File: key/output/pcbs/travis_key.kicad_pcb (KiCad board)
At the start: 2 copper layers, 38.1 x 38.1 mm, 4 parts

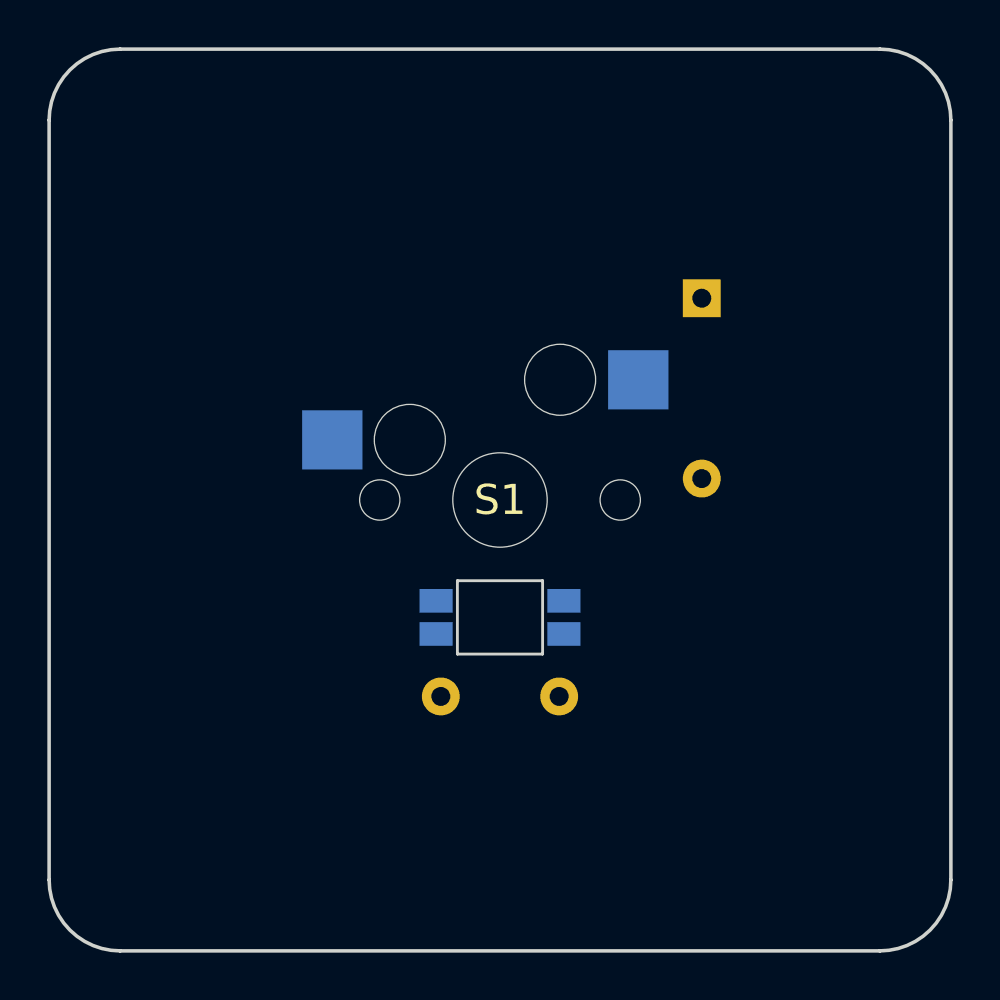
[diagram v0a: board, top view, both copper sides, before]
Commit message: footprint wip
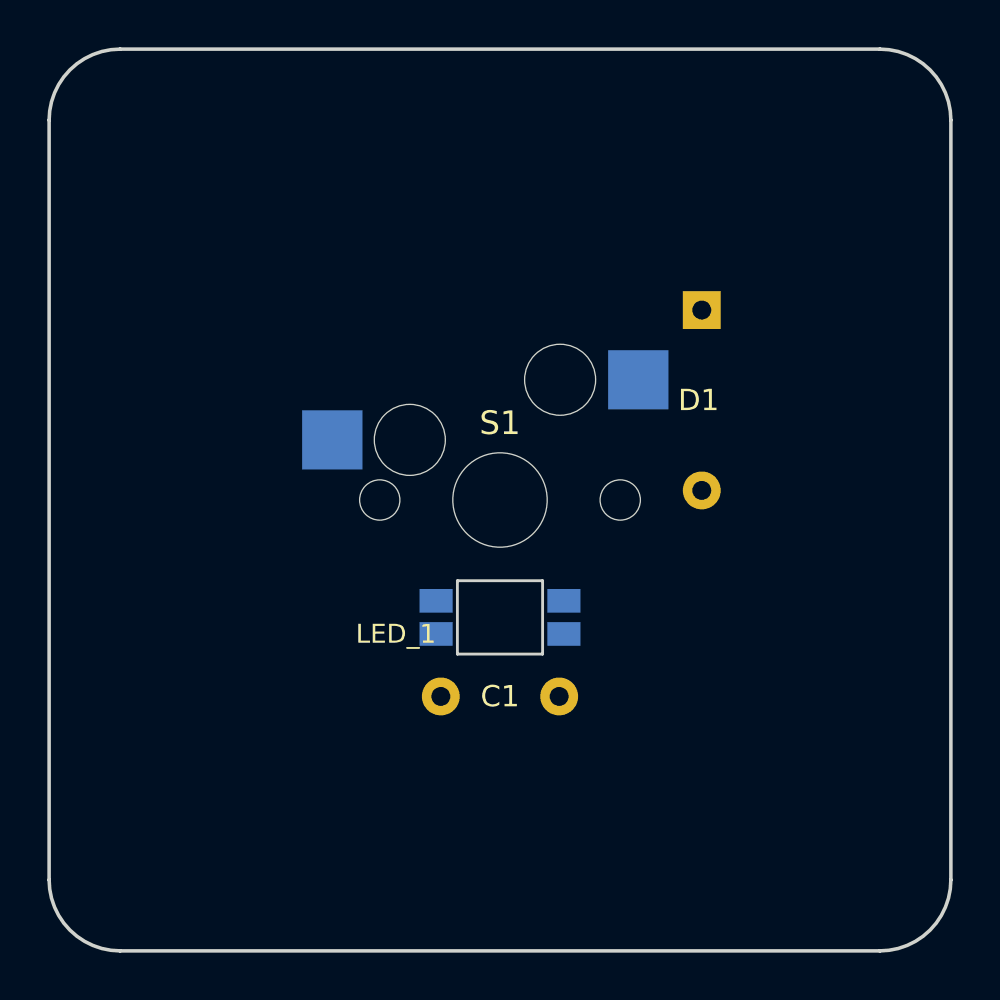
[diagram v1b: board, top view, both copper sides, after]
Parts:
- LED1: value (none) -> SK6812mini-e; footprint ceoloide:led_SK6812mini-e (per-keysingle-side) -> ceoloide:led_SK6812mini-e (per-key single-side)
- S1: value (none) -> Kailh MX Switch Sockets
- moved D1 0.50 mm to (8.53, -8.03)
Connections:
- net LED_0 renamed LED_2
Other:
- board text added: "C1"
- board text added: "D1"
- board text added: "LED_1"
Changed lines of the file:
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@@
   (title_block
     (title travis_key)
-    (rev 2024.03.20)
+    (rev 2024.03.23)
     (company "Travis Hardiman")
   )
@@
 (net 3 "row0")
 (net 4 "RAW")
-(net 5 "LED_0")
+(net 5 "LED_2")
 (net 6 "GND")
 (net 7 "LED_1")
@@
 (add_net "row0")
 (add_net "RAW")
-(add_net "LED_0")
+(add_net "LED_2")
 (add_net "GND")
 (add_net "LED_1")
   )
-      (module MX (layer F.Cu)
-      (at 0 0 0)
-      (fp_text reference "S1" (at 0 0) (layer F.SilkS)  (effects (font (size 1.27 1.27) (thickness 0.15))))
-      (fp_text value "" (at 0 0) (layer F.SilkS) hide (effects (font (size 1.27 1.27) (thickness 0.15))))
-      (fp_line (start -7 -6) (end -7 -7) (layer Dwgs.User) (width 0.15))
-      (fp_line (start -7 7) (end -6 7) (layer Dwgs.User) (width 0.15))
-      (fp_line (start -6 -7) (end -7 -7) (layer Dwgs.User) (width 0.15))
-      (fp_line (start -7 7) (end -7 6) (layer Dwgs.User) (width 0.15))
-      (fp_line (start 7 6) (end 7 7) (layer Dwgs.User) (width 0.15))
-      (fp_line (start 7 -7) (end 6 -7) (layer Dwgs.User) (width 0.15))
-      (fp_line (start 6 7) (end 7 7) (layer Dwgs.User) (width 0.15))
-      (fp_line (start 7 -7) (end 7 -6) (layer Dwgs.User) (width 0.15))
-      (pad "" np_thru_hole circle (at 0 0) (size 3.9878 3.9878) (drill 3.9878) (layers *.Cu *.Mask))
-      (pad "" np_thru_hole circle (at 5.08 0) (size 1.7018 1.7018) (drill 1.7018) (layers *.Cu *.Mask))
-      (pad "" np_thru_hole circle (at -5.08 0) (size 1.7018 1.7018) (drill 1.7018) (layers *.Cu *.Mask))
-      (fp_line (start -9.5 -9.5) (end 9.5 -9.5) (layer Dwgs.User) (width 0.15))
-      (fp_line (start 9.5 -9.5) (end 9.5 9.5) (layer Dwgs.User) (width 0.15))
-      (fp_line (start 9.5 9.5) (end -9.5 9.5) (layer Dwgs.User) (width 0.15))
-      (fp_line (start -9.5 9.5) (end -9.5 -9.5) (layer Dwgs.User) (width 0.15))
-        (pad "" np_thru_hole circle (at 2.54 -5.08) (size 3 3) (drill 3) (layers *.Cu *.Mask))
-        (pad "" np_thru_hole circle (at -3.81 -2.54) (size 3 3) (drill 3) (layers *.Cu *.Mask))
-        (pad 1 smd rect (at -7.085 -2.54 0) (size 2.55 2.5) (layers B.Cu B.Paste B.Mask) (net 1 "col0"))
-        (pad 2 smd rect (at 5.842 -5.08 0) (size 2.55 2.5) (layers B.Cu B.Paste B.Mask) (net 2 "single_A_one"))
-        )
+        (module MX (layer F.Cu)
+        (at 0 0 0)
+        (fp_text reference "S1" (at 0 -3.25) (layer F.SilkS)  (effects (font (size 1 1) (thickness 0.15))))
+        (fp_text value "Kailh MX Switch Sockets" (at 0 0) (layer B.Fab) hide (effects (font (size 1 1) (thickness 0.15))))
+        (fp_line (start -7 -6) (end -7 -7) (layer Dwgs.User) (width 0.15))
+        (fp_line (start -7 7) (end -6 7) (layer Dwgs.User) (width 0.15))
+        (fp_line (start -6 -7) (end -7 -7) (layer Dwgs.User) (width 0.15))
+        (fp_line (start -7 7) (end -7 6) (layer Dwgs.User) (width 0.15))
+        (fp_line (start 7 6) (end 7 7) (layer Dwgs.User) (width 0.15))
+        (fp_line (start 7 -7) (end 6 -7) (layer Dwgs.User) (width 0.15))
+        (fp_line (start 6 7) (end 7 7) (layer Dwgs.User) (width 0.15))
+        (fp_line (start 7 -7) (end 7 -6) (layer Dwgs.User) (width 0.15))
+        (pad "" np_thru_hole circle (at 0 0) (size 3.9878 3.9878) (drill 3.9878) (layers *.Cu *.Mask))
+        (pad "" np_thru_hole circle (at 5.08 0) (size 1.7018 1.7018) (drill 1.7018) (layers *.Cu *.Mask))
+        (pad "" np_thru_hole circle (at -5.08 0) (size 1.7018 1.7018) (drill 1.7018) (layers *.Cu *.Mask))
+        (fp_line (start -9.5 -9.5) (end 9.5 -9.5) (layer Dwgs.User) (width 0.15))
+        (fp_line (start 9.5 -9.5) (end 9.5 9.5) (layer Dwgs.User) (width 0.15))
+        (fp_line (start 9.5 9.5) (end -9.5 9.5) (layer Dwgs.User) (width 0.15))
+        (fp_line (start -9.5 9.5) (end -9.5 -9.5) (layer Dwgs.User) (width 0.15))
+          (pad "" np_thru_hole circle (at 2.54 -5.08) (size 3 3) (drill 3) (layers *.Cu *.Mask))
+          (pad "" np_thru_hole circle (at -3.81 -2.54) (size 3 3) (drill 3) (layers *.Cu *.Mask))
+          (pad 1 smd rect (at -7.085 -2.54 0) (size 2.55 2.5) (layers B.Cu B.Paste B.Mask) (net 1 "col0"))
+          (pad 2 smd rect (at 5.842 -5.08 0) (size 2.55 2.5) (layers B.Cu B.Paste B.Mask) (net 2 "single_A_one"))
+      (model "${SCOTTOKEEBS_KICAD}/3dmodels/ScottoKeebs_Hotswap.3dshapes/Hotswap_MX.step"
+		(offset (xyz 0 0 0) )
+		(scale (xyz 1 1 1) )
+		(rotate (xyz 0 0 0) )
+	  ))
     (module "Diode_DO-35" (layer "B.Cu")
     (descr "Diode, DO-35_SOD27 series, Axial, Horizontal, pin pitch=7.62mm, , length*diameter=4*2mm^2, , http://www.diodes.com/_files/packages/DO-35.pdf")
     (tags "Diode DO-35_SOD27 series Axial Horizontal pin pitch 7.62mm  length 4mm diameter 2mm")
-    (at 8.525 -8.525 270)
-    (fp_text reference "D1" (at 3.81 -2.12 270) (layer "B.SilkS")
+    (at 8.525 -8.025 270)
+    (fp_text reference "D1" (at 5.985 1.921 270) (layer "B.SilkS")
       (effects (font (size 1 1) (thickness 0.15)) (justify mirror))
     )
-    (fp_text value "1N4148" (at 3.81 0 270) (layer "B.Fab")
-      (effects (font (size 0.8 1) (thickness 0.15)))
-    )
-    (fp_text user "K" (at 0 -1.8 270) (layer "B.SilkS")
-      (effects (font (size 1 1) (thickness 0.15)) (justify mirror))
-    )
-    (fp_text user "K" (at 0 -1.8 270) (layer "B.Fab")
-      (effects (font (size 1 1) (thickness 0.15)) (justify mirror))
+    (fp_text value "1N4148" (at 11.065 0 270) (layer "B.Fab")
+      (effects (font (size 0.8 0.8) (thickness 0.15)))
     )
     (fp_line (start 1.04 0) (end 1.69 0)
@@
     )
   )
-      (module "ceoloide:led_SK6812mini-e (per-keysingle-side)"
+      (gr_text "D1" (at 7.525 -4.215 0) (layer F.SilkS)
+        (effects (font (size 0.9 0.9) (thickness 0.15)) (justify left))
+      )
+      (module "ceoloide:led_SK6812mini-e (per-key single-side)"
         (layer B.Cu)
         (at 0 4.96 0)
-        (fp_text reference "LED1" (at -4.75 0 90) (layer B.SilkS)
-          (effects (font (size 1 1) (thickness 0.15)))
+        (fp_text reference "LED1" (at -5.25 0 90) (layer B.SilkS)
+          (effects (font (size 1 1) (thickness 0.15)) (justify  mirror))
+        )
+        (fp_text value "SK6812mini-e" (at 0 -2.25 0) (layer "B.Fab")
+          (effects (font (size 0.8 0.8) (thickness 0.15)))
         )
         (fp_line (start -1.6 -1.4) (end 1.6 -1.4) (layer Dwgs.User) (width 0.12))
@@
         (fp_line (start -3.8 -1.6) (end -2.2 -1.6) (layer B.SilkS) (width 0.12))
         (fp_line (start -3.8 0) (end -3.8 -1.6) (layer B.SilkS) (width 0.12))
-        (pad 2 smd rect (at 2.70 -0.7 0) (size 1.4 1) (layers B.Cu B.Paste B.Mask) (net 5 "LED_0"))
+        (fp_line (start -3.8 -1.36) (end -3.56 -1.6) (layer B.SilkS) (width 0.12))
+        (pad 2 smd rect (at 2.70 -0.7 0) (size 1.4 1) (layers B.Cu B.Paste B.Mask) (net 5 "LED_2"))
         (pad 1 smd rect (at 2.70 0.7 0) (size 1.4 1) (layers B.Cu B.Paste B.Mask) (net 4 "RAW"))
         (pad 3 smd rect (at -2.70 -0.7 0) (size 1.4 1) (layers B.Cu B.Paste B.Mask) (net 6 "GND"))
@@
         )
       )
+      (gr_text "LED_1" (at -2.7 5.66 0) (layer F.SilkS)
+        (effects (font (size 0.8 0.8) (thickness 0.15)) (justify right))
+      )
     (module C_Disc_D4.7mm_W2.5mm_P5.00mm (layer B.Cu)
     (descr "C, Disc series, Radial, pin pitch=5.00mm, , diameter*width=4.7*2.5mm^2, Capacitor, http://www.vishay.com/docs/45233/krseries.pdf")
     (tags "C Disc series Radial pin pitch 5.00mm  diameter 4.7mm width 2.5mm Capacitor")
     (at 2.5 8.3 180)
-    (fp_text reference "C1" (at 2.5 -2.5 180) (layer B.SilkS)
+    (fp_text reference "C1" (at 7.5 0 180) (layer B.SilkS)
       (effects (font (size 1 1) (thickness 0.15)) (justify mirror))
     )
-    (fp_text value "104" (at 2.5 2.5 180) (layer B.Fab)
+    (fp_text value "104" (at -2.5 0 180) (layer B.Fab)
       (effects (font (size 1 1) (thickness 0.15)))
     )
@@
     (pad 1 thru_hole circle (at 0 0) (size 1.6 1.6) (drill 0.8) (layers *.Cu *.Mask) (net 4 "RAW"))
     (pad 2 thru_hole circle (at 5 0) (size 1.6 1.6) (drill 0.8) (layers *.Cu *.Mask) (net 6 "GND"))
-    (fp_text user %R (at 2.5 0) (layer B.Fab)
-      (effects (font (size 0.94 0.94) (thickness 0.141)))
-    )
     (model ${KISYS3DMOD}/Capacitor_THT.3dshapes/C_Disc_D4.7mm_W2.5mm_P5.00mm.wrl
       (at (xyz 0 0 0))
@@
     )
   )
+      (gr_text "C1" (at 0 8.3 0) (layer F.SilkS)
+        (effects (font (size 0.9 0.9) (thickness 0.15)))
+      )
             (gr_line (start -19.05 16.05) (end -19.05 -16.05) (angle 90) (layer Edge.Cuts) (width 0.15))
 (gr_line (start -16.05 -19.05) (end 16.05 -19.05) (angle 90) (layer Edge.Cuts) (width 0.15))
